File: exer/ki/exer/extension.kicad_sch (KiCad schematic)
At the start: 6 parts, among them J1 Conn_01x20, J2 Conn_01x20, J3 Conn_01x34, J4 Conn_01x34, U10 74HCT574, U11 74HCT574

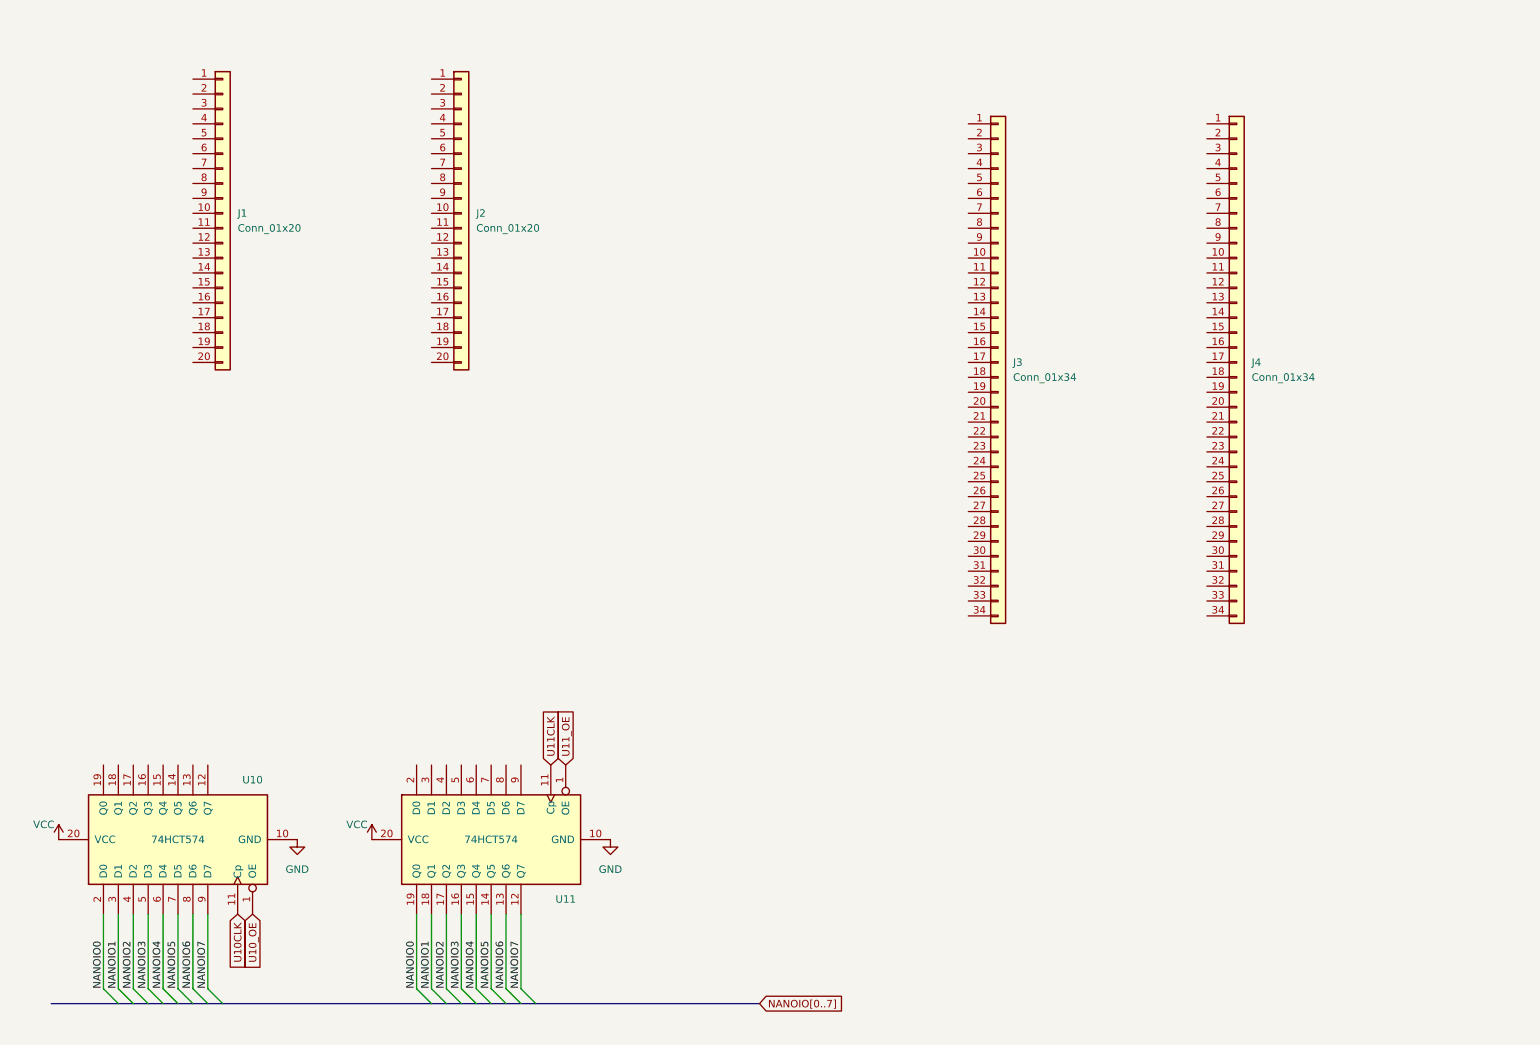
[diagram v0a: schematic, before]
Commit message: Ongoing development
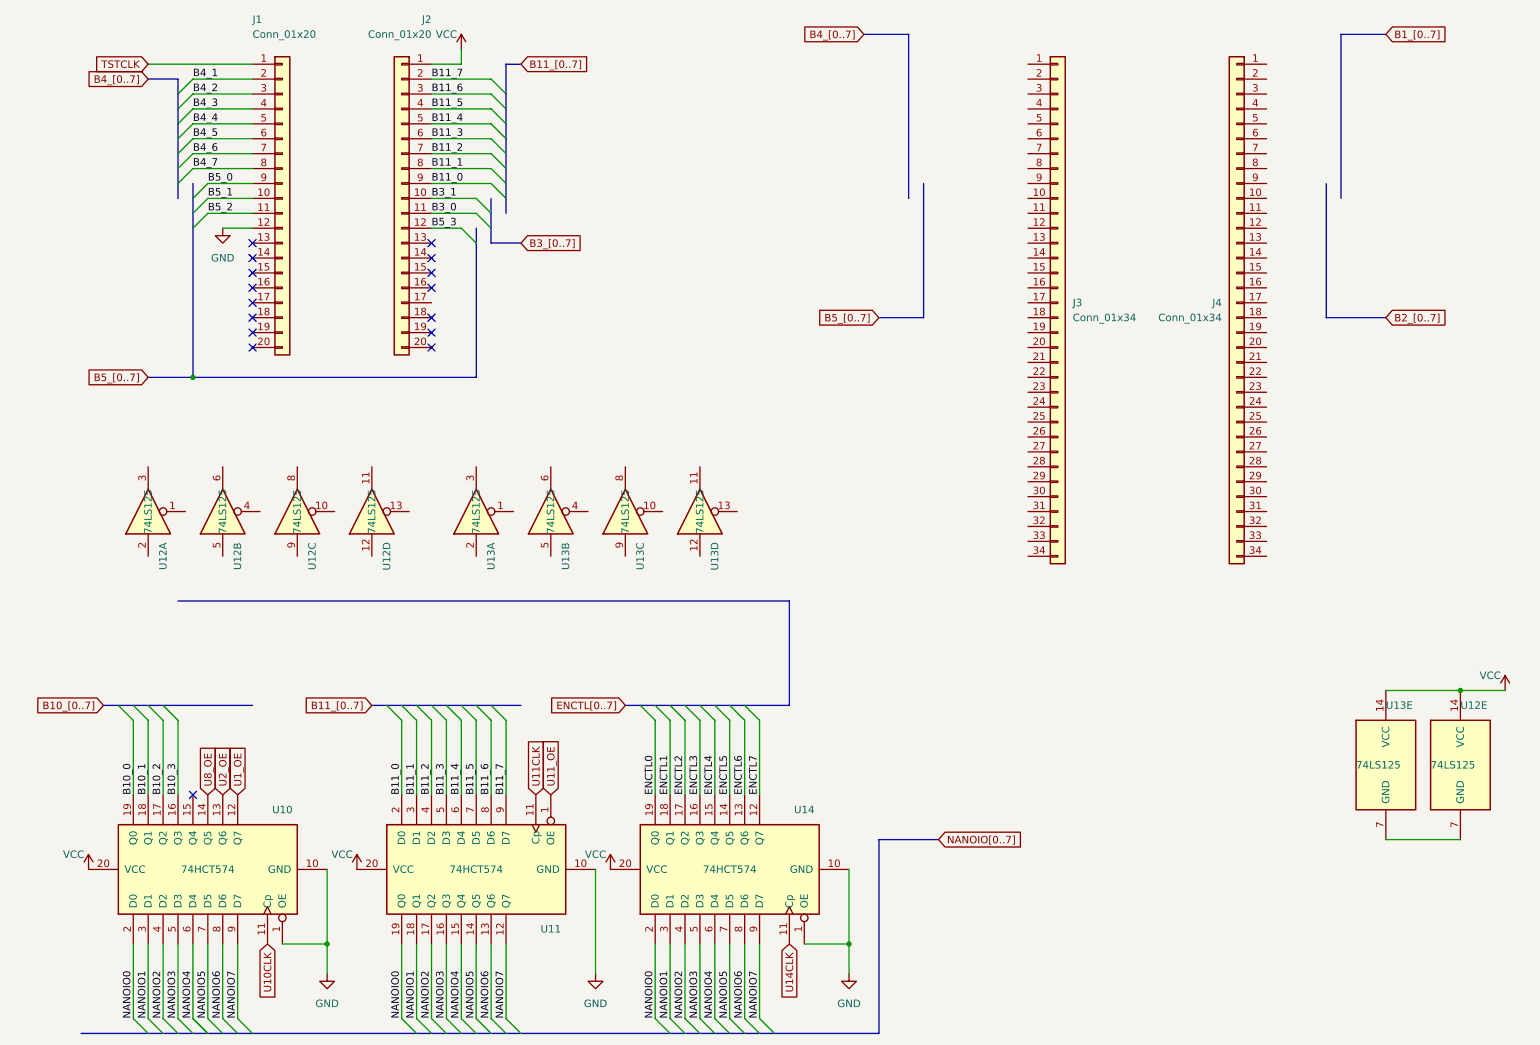
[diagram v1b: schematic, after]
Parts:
- added U12, U13: 74LS125, symbol 74xx:74LS125
- added U14: 74HCT574, symbol 74xx:74HCT574
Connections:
- net U10_OE is gone; now on net GND: U10.1 (OE)
- net GND: now also J1.12 (Pin_12), U14.1 (OE), U14.10 (GND)
- net NANOIO0: now also U14.2 (D0)
- net NANOIO1: now also U14.3 (D1)
- net NANOIO2: now also U14.4 (D2)
- net NANOIO3: now also U14.5 (D3)
- net NANOIO4: now also U14.6 (D4)
- net NANOIO5: now also U14.7 (D5)
- net NANOIO6: now also U14.8 (D6)
- net NANOIO7: now also U14.9 (D7)
- net VCC: now also J2.1 (Pin_1), U12.14 (VCC), U13.14 (VCC), U14.20 (VCC)
- net TSTCLK: now reaches J1.1 (Pin_1)
- net B5_1: now reaches J1.10 (Pin_10)
- net B5_2: now reaches J1.11 (Pin_11)
- net B4_1: now reaches J1.2 (Pin_2)
- net B4_2: now reaches J1.3 (Pin_3)
- net B4_3: now reaches J1.4 (Pin_4)
- net B4_4: now reaches J1.5 (Pin_5)
- net B4_5: now reaches J1.6 (Pin_6)
- net B4_6: now reaches J1.7 (Pin_7)
- net B4_7: now reaches J1.8 (Pin_8)
- net B5_0: now reaches J1.9 (Pin_9)
- net U1_OE: now reaches U10.12 (Q7)
- net U2_OE: now reaches U10.13 (Q6)
- net U8_OE: now reaches U10.14 (Q5)
- net B10_3: now reaches U10.16 (Q3)
- net B10_2: now reaches U10.17 (Q2)
- net B10_1: now reaches U10.18 (Q1)
- net B10_0: now reaches U10.19 (Q0)
- net B11_0: now reaches U11.2 (D0)
- net B11_0: now also J2.9 (Pin_9)
- net B11_1: now reaches U11.3 (D1)
- net B11_1: now also J2.8 (Pin_8)
- net B11_2: now reaches U11.4 (D2)
- net B11_2: now also J2.7 (Pin_7)
- net B11_3: now reaches U11.5 (D3)
- net B11_3: now also J2.6 (Pin_6)
- net B11_4: now reaches U11.6 (D4)
- net B11_4: now also J2.5 (Pin_5)
- net B11_5: now reaches U11.7 (D5)
- net B11_5: now also J2.4 (Pin_4)
- net B11_6: now reaches U11.8 (D6)
- net B11_6: now also J2.3 (Pin_3)
- net B11_7: now reaches U11.9 (D7)
- net B11_7: now also J2.2 (Pin_2)
- net B3_1: now reaches J2.10 (Pin_10)
- net B3_0: now reaches J2.11 (Pin_11)
- net B5_3: now reaches J2.12 (Pin_12)
- new net: U12.7 (GND), U13.7 (GND)
- new net ENCTL0: U14.19 (Q0)
- new net ENCTL1: U14.18 (Q1)
- new net ENCTL2: U14.17 (Q2)
- new net ENCTL3: U14.16 (Q3)
- new net ENCTL4: U14.15 (Q4)
- new net ENCTL5: U14.14 (Q5)
- new net ENCTL6: U14.13 (Q6)
- new net ENCTL7: U14.12 (Q7)
- new net U14CLK: U14.11 (Cp)
- no-connect marks 0 -> 16
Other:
- moved on the sheet: J1, J2, J3, J4, U10, U11

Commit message: Ongoing development of chip exerciser
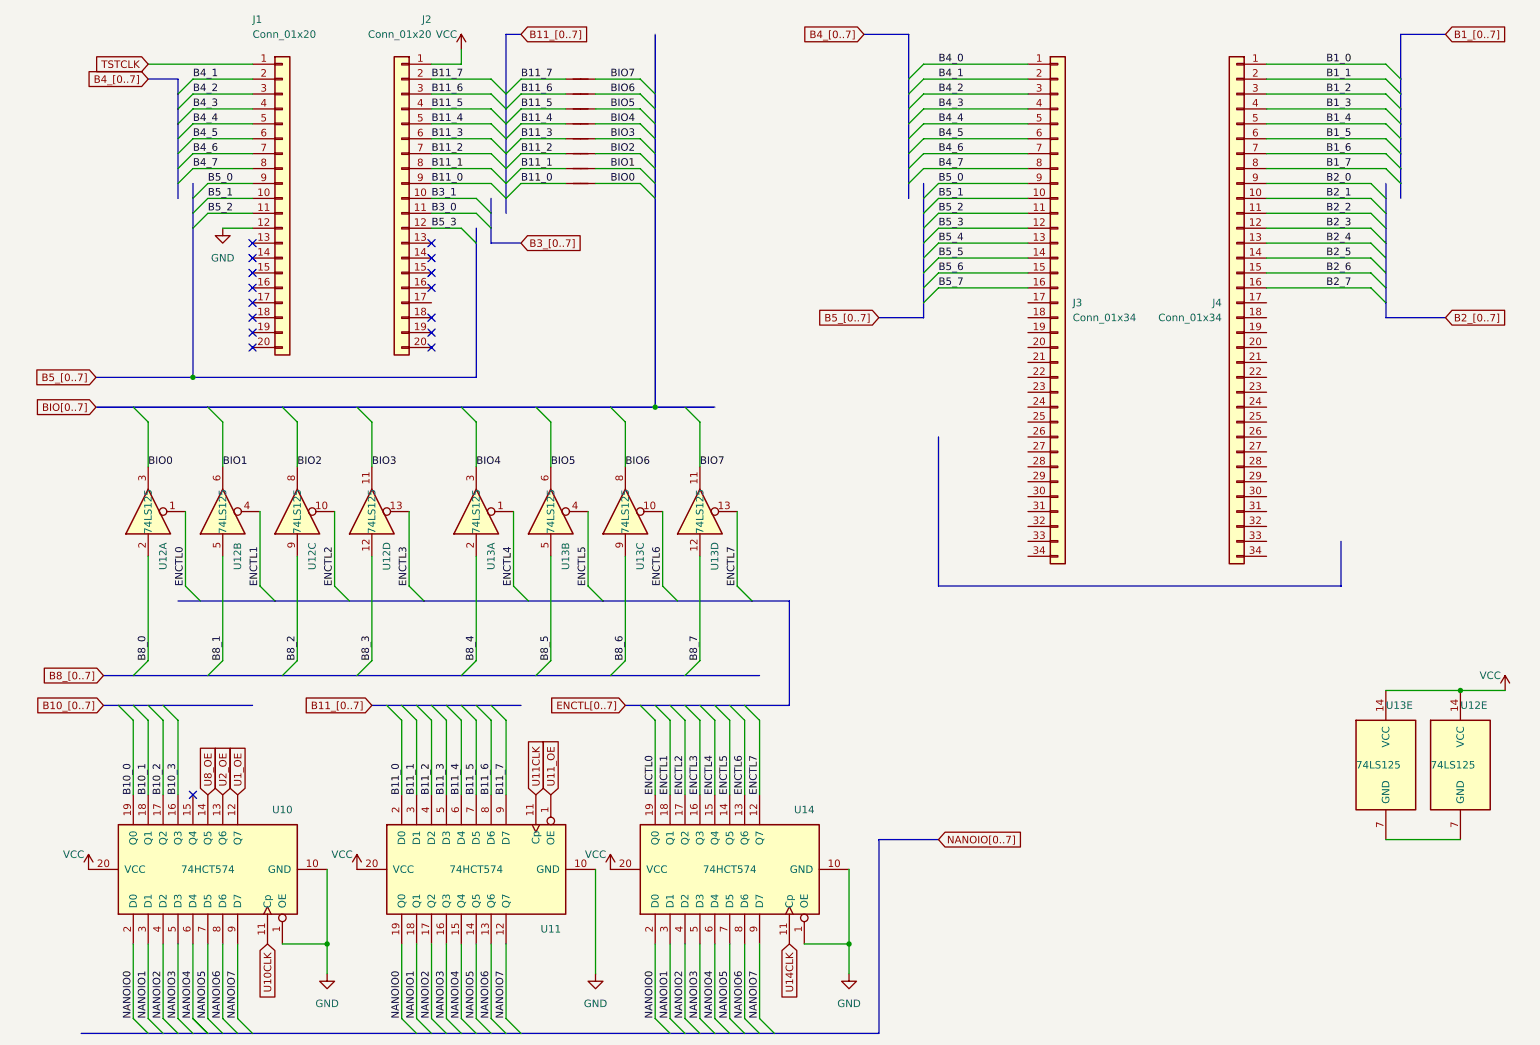
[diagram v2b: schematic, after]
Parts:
- added NT1, NT2, NT3, NT4, NT5, NT6, NT7, NT8: NetTie_2, symbol Device:NetTie_2
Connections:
- net B11_0: now also NT8.1
- net B11_1: now also NT7.1
- net B11_2: now also NT6.1
- net B11_3: now also NT5.1
- net B11_4: now also NT4.1
- net B11_5: now also NT3.1
- net B11_6: now also NT2.1
- net B11_7: now also NT1.1
- net B4_1: now also J3.2 (Pin_2)
- net B4_2: now also J3.3 (Pin_3)
- net B4_3: now also J3.4 (Pin_4)
- net B4_4: now also J3.5 (Pin_5)
- net B4_5: now also J3.6 (Pin_6)
- net B4_6: now also J3.7 (Pin_7)
- net B4_7: now also J3.8 (Pin_8)
- net B5_0: now also J3.9 (Pin_9)
- net B5_1: now also J3.10 (Pin_10)
- net B5_2: now also J3.11 (Pin_11)
- net B5_3: now also J3.12 (Pin_12)
- net ENCTL0: now also U12.1
- net ENCTL1: now also U12.4
- net ENCTL2: now also U12.10
- net ENCTL3: now also U12.13
- net ENCTL4: now also U13.1
- net ENCTL5: now also U13.4
- net ENCTL6: now also U13.10
- net ENCTL7: now also U13.13
- net BIO6: now reaches U13.8
- net BIO6: now also NT2.2
- net B8_6: now reaches U13.9
- net BIO3: now reaches U12.11
- net BIO3: now also NT5.2
- net B8_3: now reaches U12.12
- net BIO7: now reaches U13.11
- net BIO7: now also NT1.2
- net B8_7: now reaches U13.12
- net B8_4: now reaches U13.2
- net BIO4: now reaches U13.3
- net BIO4: now also NT4.2
- net B8_5: now reaches U13.5
- net BIO5: now reaches U13.6
- net BIO5: now also NT3.2
- net B8_1: now reaches U12.5
- net BIO1: now reaches U12.6
- net BIO1: now also NT7.2
- net B1_0: now reaches J4.1 (Pin_1)
- net B2_1: now reaches J4.10 (Pin_10)
- net B2_2: now reaches J4.11 (Pin_11)
- net B2_3: now reaches J4.12 (Pin_12)
- net B2_4: now reaches J4.13 (Pin_13)
- net B2_5: now reaches J4.14 (Pin_14)
- net B2_6: now reaches J4.15 (Pin_15)
- net B2_7: now reaches J4.16 (Pin_16)
- net B1_1: now reaches J4.2 (Pin_2)
- net B1_2: now reaches J4.3 (Pin_3)
- net B1_3: now reaches J4.4 (Pin_4)
- net B1_4: now reaches J4.5 (Pin_5)
- net B1_5: now reaches J4.6 (Pin_6)
- net B1_6: now reaches J4.7 (Pin_7)
- net B1_7: now reaches J4.8 (Pin_8)
- net B2_0: now reaches J4.9 (Pin_9)
- net BIO2: now reaches U12.8
- net BIO2: now also NT6.2
- net B8_2: now reaches U12.9
- net B8_0: now reaches U12.2
- net BIO0: now reaches U12.3
- net BIO0: now also NT8.2
- net B4_0: now reaches J3.1 (Pin_1)
- net B5_4: now reaches J3.13 (Pin_13)
- net B5_5: now reaches J3.14 (Pin_14)
- net B5_6: now reaches J3.15 (Pin_15)
- net B5_7: now reaches J3.16 (Pin_16)

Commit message: Hardware design roughly complete
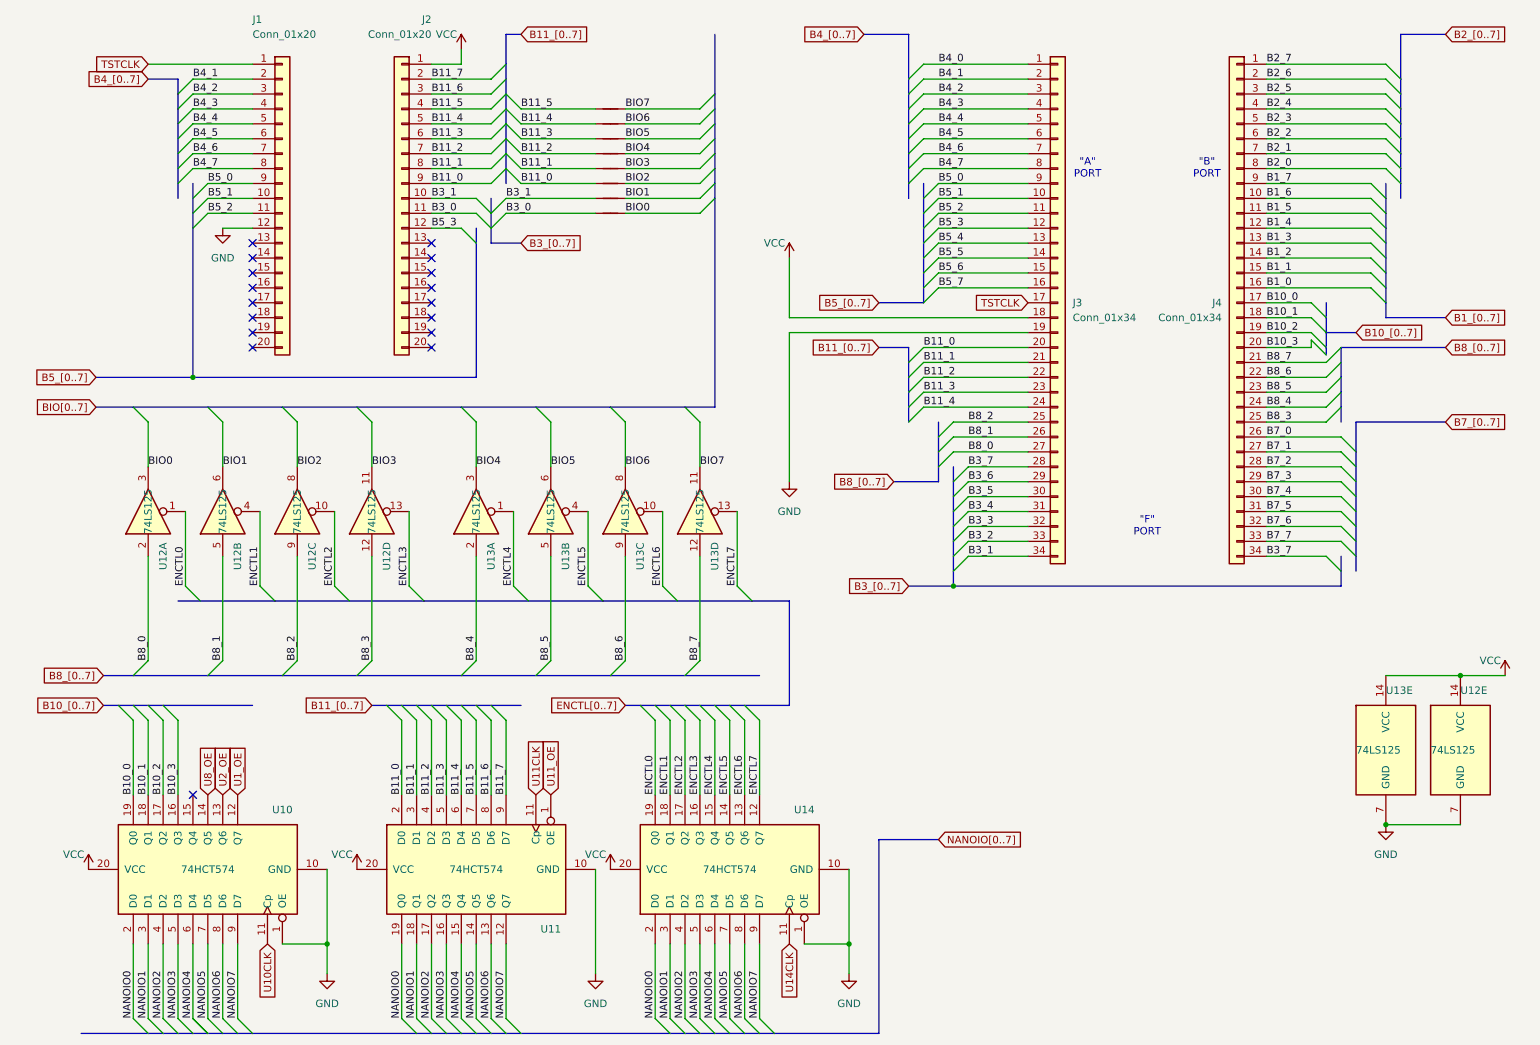
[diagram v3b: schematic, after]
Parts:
- removed NT7, NT8: NetTie_2, symbol Device:NetTie_2
- added NT15, NT16: NetTie_2, symbol Device:NetTie_2
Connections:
- net B10_0: now also J4.17 (Pin_17)
- net B10_1: now also J4.18 (Pin_18)
- net B10_2: now also J4.19 (Pin_19)
- net B10_3: now also J4.20 (Pin_20)
- net B11_0: now also J3.20 (Pin_20), NT6.1
- net B11_1: now also J3.21 (Pin_21), NT5.1
- net B11_2: now also J3.22 (Pin_22), NT4.1; no longer NT6.1
- net B11_3: now also J3.23 (Pin_23), NT3.1; no longer NT5.1
- net B11_4: now also J3.24 (Pin_24), NT2.1; no longer NT4.1
- net B11_5: now also NT1.1; no longer NT3.1
- net B11_6: no longer NT2.1
- net B11_7: no longer NT1.1
- net B1_0: now also J4.16 (Pin_16); no longer J4.1 (Pin_1)
- net B1_1: now also J4.15 (Pin_15); no longer J4.2 (Pin_2)
- net B1_2: now also J4.14 (Pin_14); no longer J4.3 (Pin_3)
- net B1_3: now also J4.13 (Pin_13); no longer J4.4 (Pin_4)
- net B1_4: now also J4.12 (Pin_12); no longer J4.5 (Pin_5)
- net B1_5: now also J4.11 (Pin_11); no longer J4.6 (Pin_6)
- net B1_6: now also J4.10 (Pin_10); no longer J4.7 (Pin_7)
- net B1_7: now also J4.9 (Pin_9); no longer J4.8 (Pin_8)
- net B2_0: now also J4.8 (Pin_8); no longer J4.9 (Pin_9)
- net B2_1: now also J4.7 (Pin_7); no longer J4.10 (Pin_10)
- net B2_2: now also J4.6 (Pin_6); no longer J4.11 (Pin_11)
- net B2_3: now also J4.5 (Pin_5); no longer J4.12 (Pin_12)
- net B2_4: now also J4.4 (Pin_4); no longer J4.13 (Pin_13)
- net B2_5: now also J4.3 (Pin_3); no longer J4.14 (Pin_14)
- net B2_6: now also J4.2 (Pin_2); no longer J4.15 (Pin_15)
- net B2_7: now also J4.1 (Pin_1); no longer J4.16 (Pin_16)
- net B3_0: now also NT16.1
- net B3_1: now also J3.34 (Pin_34), NT15.1
- net B8_0: now also J3.27 (Pin_27)
- net B8_1: now also J3.26 (Pin_26)
- net B8_2: now also J3.25 (Pin_25)
- net B8_3: now also J4.25 (Pin_25)
- net B8_4: now also J4.24 (Pin_24)
- net B8_5: now also J4.23 (Pin_23)
- net B8_6: now also J4.22 (Pin_22)
- net B8_7: now also J4.21 (Pin_21)
- net BIO0: now also NT16.2
- net BIO1: now also NT15.2
- net GND: now also J3.19 (Pin_19), U12.7 (GND), U13.7 (GND)
- net TSTCLK: now also J3.17 (Pin_17)
- net VCC: now also J3.18 (Pin_18)
- net B7_0: now reaches J4.26 (Pin_26)
- net B7_1: now reaches J4.27 (Pin_27)
- net B7_2: now reaches J4.28 (Pin_28)
- net B7_3: now reaches J4.29 (Pin_29)
- net B7_4: now reaches J4.30 (Pin_30)
- net B7_5: now reaches J4.31 (Pin_31)
- net B7_6: now reaches J4.32 (Pin_32)
- net B7_7: now reaches J4.33 (Pin_33)
- net B3_7: now reaches J4.34 (Pin_34)
- net B3_7: now also J3.28 (Pin_28)
- net B3_6: now reaches J3.29 (Pin_29)
- net B3_5: now reaches J3.30 (Pin_30)
- net B3_4: now reaches J3.31 (Pin_31)
- net B3_3: now reaches J3.32 (Pin_32)
- net B3_2: now reaches J3.33 (Pin_33)
- no-connect marks 16 -> 17
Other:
- note added: ""A" PORT"
- note added: ""B" PORT"
- note added: ""F" PORT"
- moved on the sheet: U12E, U13E
